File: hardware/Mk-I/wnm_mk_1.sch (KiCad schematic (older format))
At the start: 34 parts, among them SW1 SW_PUSH, SW10 SW_PUSH, SW11 SW_PUSH, SW12 SW_PUSH, SW13 SW_PUSH, SW14 SW_PUSH, SW15 SW_PUSH, SW16 SW_PUSH, SW18 SW_PUSH, SW19 SW_PUSH, SW2 SW_PUSH, SW20 SW_PUSH, SW21 SW_PUSH, SW22 SW_PUSH, SW3 SW_PUSH, SW4 SW_PUSH, SW5 SW_PUSH, SW6 SW_PUSH, SW7 SW_PUSH, SW8 SW_PUSH, SW9 SW_PUSH, U6 encoder_and_switch, U7 encoder_and_switch

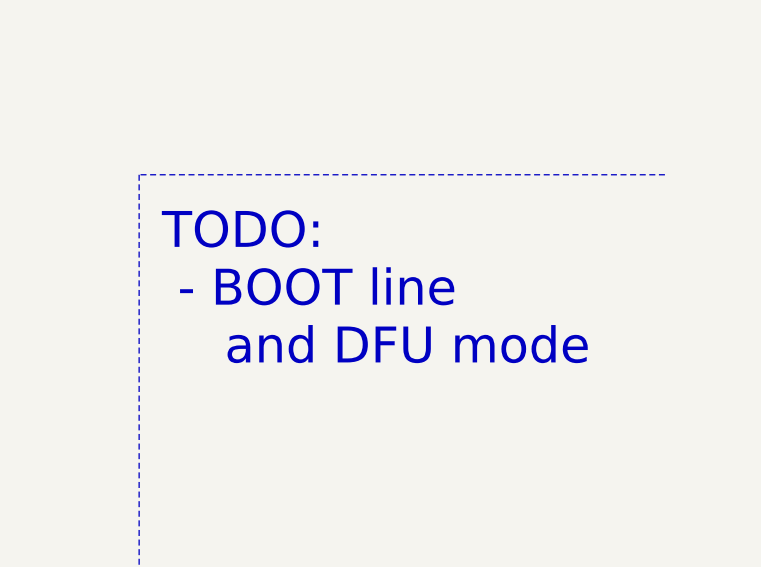
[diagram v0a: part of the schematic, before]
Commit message: HW: Update TODO list
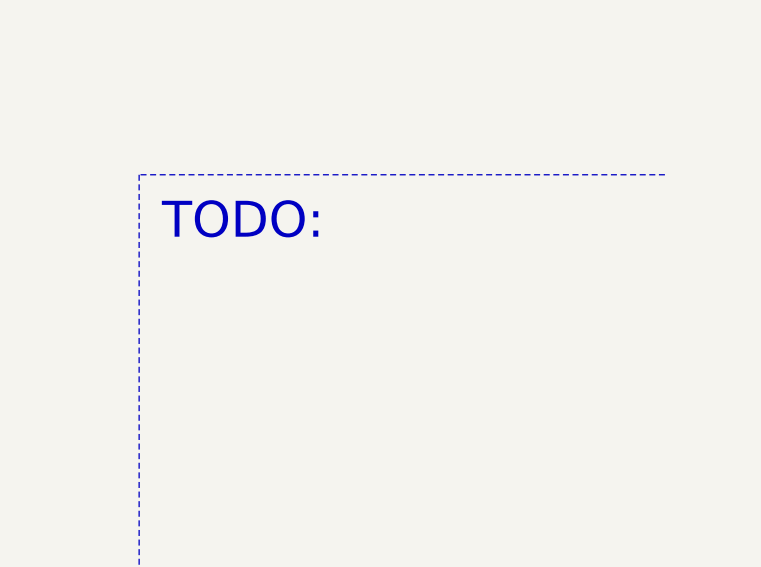
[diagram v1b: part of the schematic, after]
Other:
- note added: "TODO:"
- note removed: "TODO:\n - BOOT line \n and DFU mode"
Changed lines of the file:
@@
 F1 "audio.sch" 60
 $EndSheet
-Text Notes 8950 4950 0    157  ~ 0
-TODO:\n - BOOT line \n    and DFU mode
 Text GLabel 4850 5700 0    60   Input ~ 0
 WAKEUP
@@
 	1    0    0    -1
 $EndComp
+Text Notes 8950 4400 0    157  ~ 0
+TODO:
 $EndSCHEMATC
